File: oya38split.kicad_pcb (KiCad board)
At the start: 2 copper layers, 217.5 x 106.4 mm, 89 parts, among them U1 ProMicro

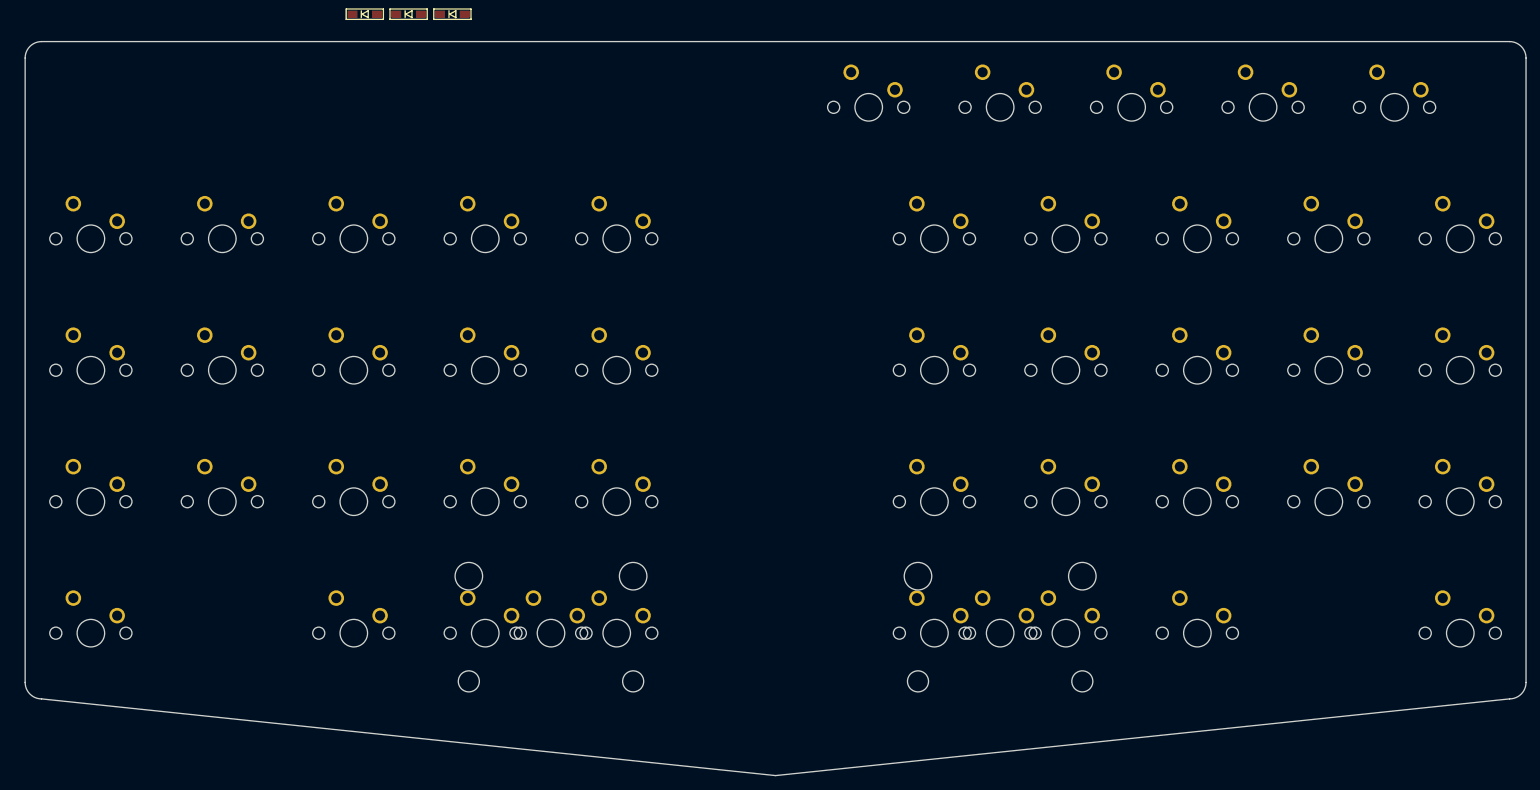
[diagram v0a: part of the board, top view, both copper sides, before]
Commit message: fixed layout
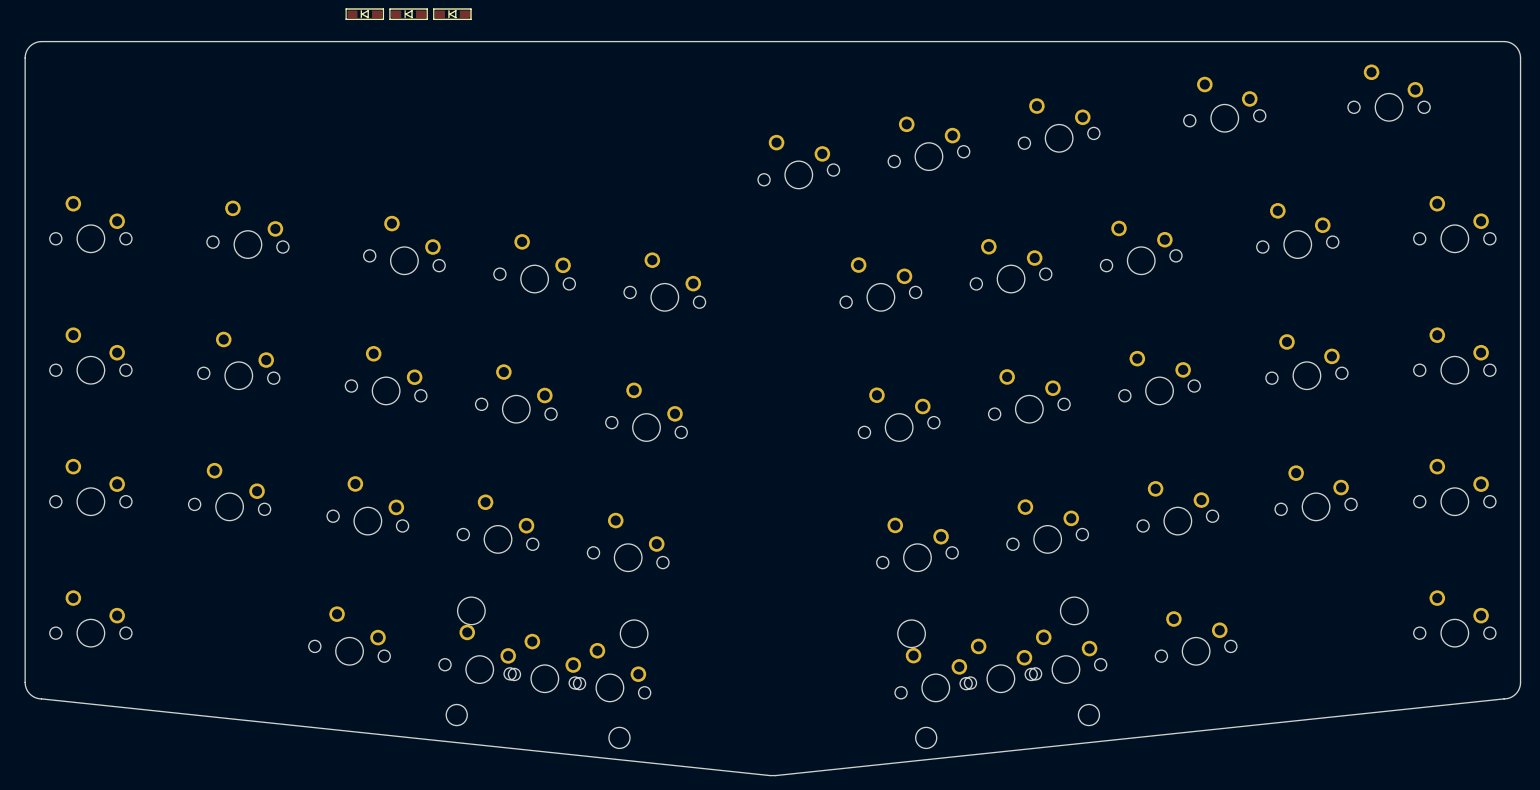
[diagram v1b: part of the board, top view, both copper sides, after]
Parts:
- moved MX39 14.1 mm to (159.7, 47.9), turned to 188 degrees
- moved MX40 12.6 mm to (178.6, 45.2), turned to 188 degrees
- moved MX6 11.5 mm to (171.6, 65.6), turned to 188 degrees
- moved MX41 11.4 mm to (197.5, 42.6), turned to 188 degrees
- moved MX5 11.0 mm to (140.3, 65.6), turned to 172 degrees
- moved MX7 9.86 mm to (190.5, 63.0), turned to 188 degrees
- moved MX16 9.75 mm to (174.3, 84.5), turned to 188 degrees
- moved MX15 9.35 mm to (137.7, 84.5), turned to 172 degrees
- moved MX4 9.23 mm to (121.5, 63.0), turned to 172 degrees
- moved MX8 8.73 mm to (209.4, 60.3), turned to 188 degrees
- moved MX26 8.48 mm to (176.9, 103.4), turned to 188 degrees
- moved MX25 8.28 mm to (135.0, 103.4), turned to 172 degrees
- moved MX3 8.00 mm to (102.6, 60.3), turned to 172 degrees
- moved MX34 7.99 mm to (132.4, 122.2), turned to 172 degrees
- moved MX35 7.93 mm to (179.6, 122.2), turned to 188 degrees
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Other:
- board size 217.5 x 106.4 mm -> 216.7 x 106.4 mm

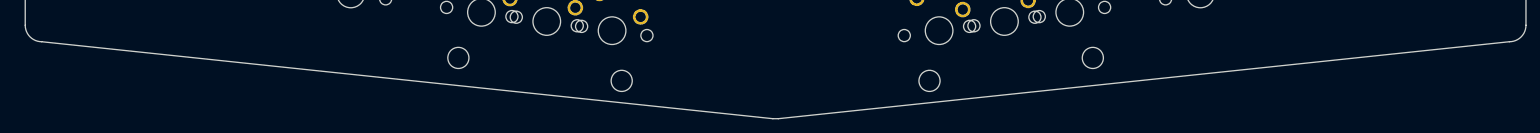
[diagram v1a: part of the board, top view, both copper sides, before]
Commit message: fixed edgecut
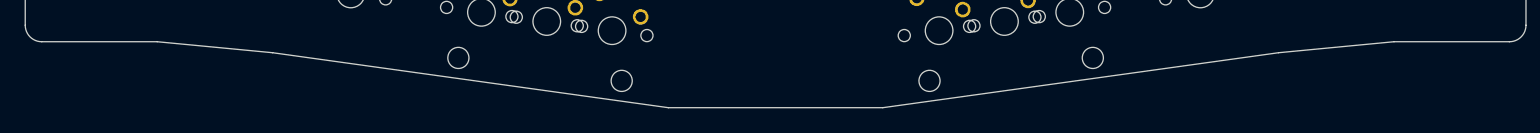
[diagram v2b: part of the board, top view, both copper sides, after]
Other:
- board size 216.7 x 106.4 mm -> 216.7 x 104.8 mm
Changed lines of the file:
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@@
   (general
     (thickness 1.6)
-    (drawings 10)
+    (drawings 14)
     (tracks 0)
     (zones 0)
@@
     )
   )
-  (gr_line (start 155.575 134.9375) (end 50.00625 123.825) (layer Edge.Cuts) (width 0.05))
-  (gr_line (start 156.36875 134.9375) (end 155.575 134.9375) (layer Edge.Cuts) (width 0.05))
-  (gr_line (start 261.9375 123.825) (end 156.36875 134.9375) (layer Edge.Cuts) (width 0.05))
+  (gr_line (start 140.49375 133.35) (end 171.45 133.35) (layer Edge.Cuts) (width 0.05))
+  (gr_line (start 83.34375 125.4125) (end 140.49375 133.35) (layer Edge.Cuts) (width 0.05))
+  (gr_line (start 66.675 123.825) (end 83.34375 125.4125) (layer Edge.Cuts) (width 0.05))
+  (gr_line (start 50.00625 123.825) (end 66.675 123.825) (layer Edge.Cuts) (width 0.05))
+  (gr_line (start 228.6 125.4125) (end 171.45 133.35) (layer Edge.Cuts) (width 0.05))
+  (gr_line (start 245.26875 123.825) (end 228.6 125.4125) (layer Edge.Cuts) (width 0.05))
+  (gr_line (start 261.9375 123.825) (end 245.26875 123.825) (layer Edge.Cuts) (width 0.05))
   (gr_line (start 50.00625 28.575) (end 261.9375 28.575) (layer Edge.Cuts) (width 0.05))
   (gr_line (start 264.31875 30.95625) (end 264.31875 121.44375) (layer Edge.Cuts) (width 0.05))
